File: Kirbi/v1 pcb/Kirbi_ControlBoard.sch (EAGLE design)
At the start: 69 parts, among them U1 PCA9306_LSSOP, U2 TEENSY_3.6_DIL, U3 MAX4173-SOT-23, U4 MAX4173-SOT-23, U5 LM393-8-SOIC, U6 AP2114H-1.8TRG1, U7 AP2114H-3.3TRG1

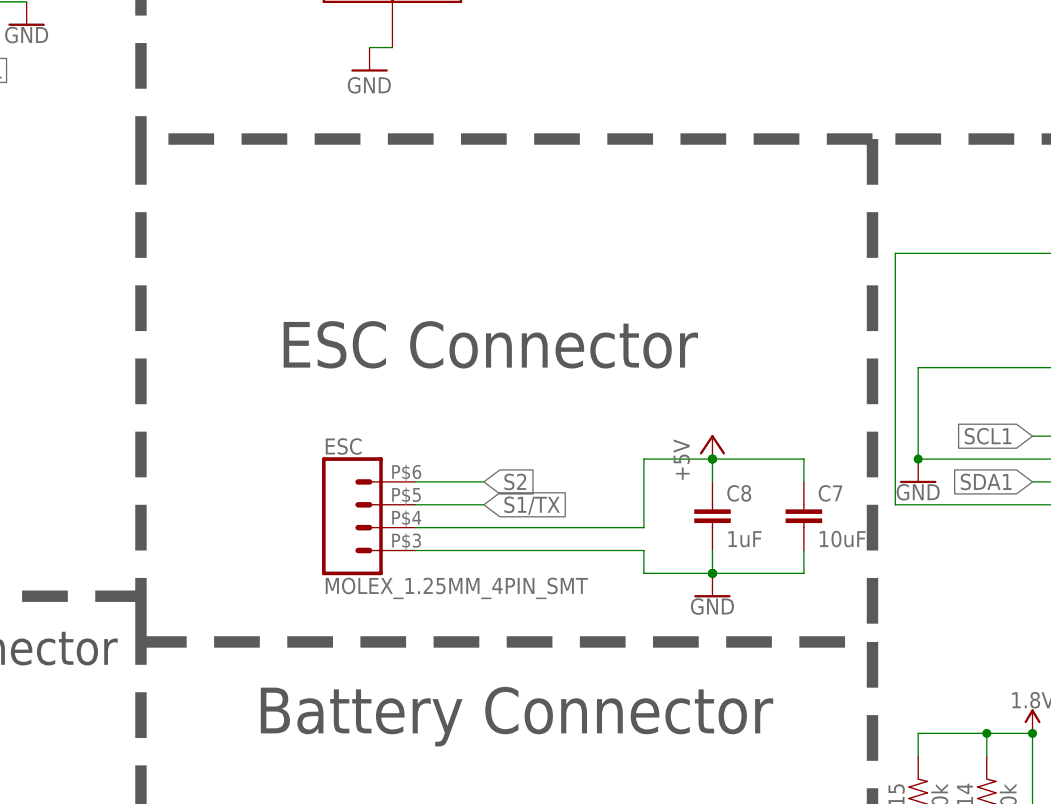
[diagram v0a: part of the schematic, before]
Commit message: Started to add power button
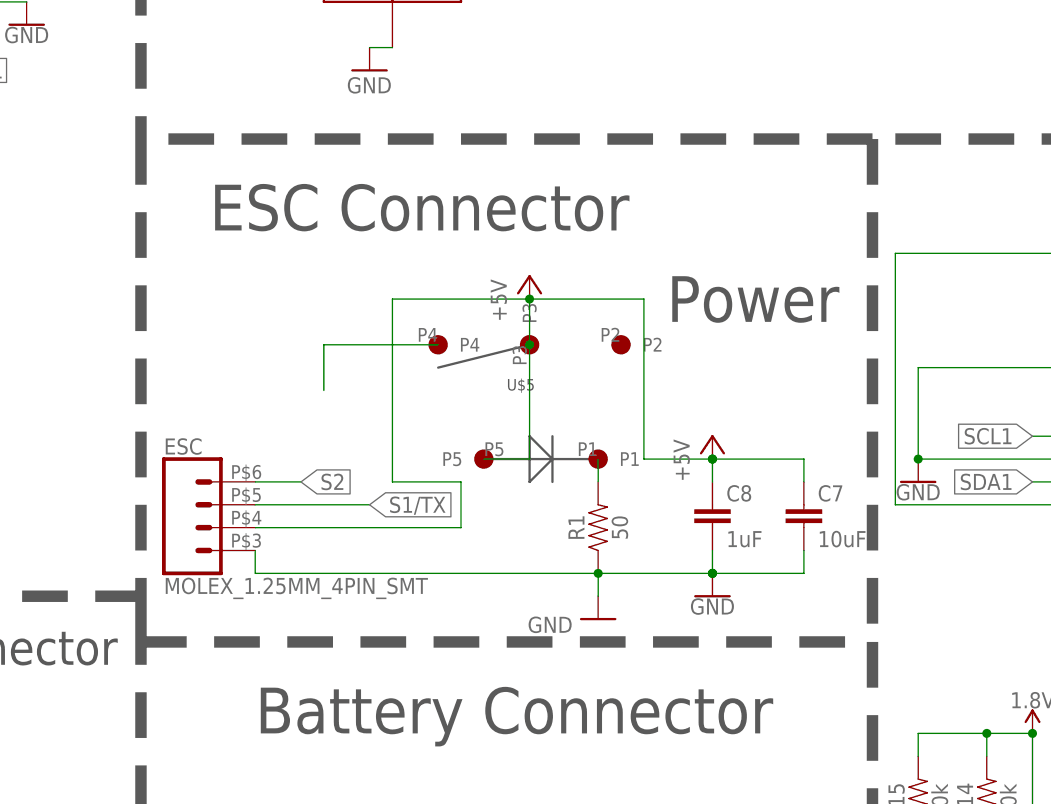
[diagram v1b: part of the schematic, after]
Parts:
- added R1: 50, SparkFun-Resistors:1KOHM-0603-1/10W-1%
- added U$5: POWER_SWITCH, Kirbi_ControlBoard:POWER_SWITCH
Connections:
- new net N$5: U$5.P4
- new net N$8: R1.2, U$5.P1
- net +5V: now also U$5.P3, U$5.P5
- net GND: now also R1.1
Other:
- note added: "Power"
- moved on the sheet: ESC
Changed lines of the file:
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@@
 <part name="LIDAR_R" library="Kirbi_ControlBoard" deviceset="MOLEX_1.25MM_4PIN_SMT" device=""/>
 <part name="LIDAR_L" library="Kirbi_ControlBoard" deviceset="MOLEX_1.25MM_4PIN_SMT" device=""/>
+<part name="U$5" library="Kirbi_ControlBoard" deviceset="POWER_SWITCH" device=""/>
+<part name="P+3" library="supply1" library_urn="urn:adsk.eagle:library:371" deviceset="+5V" device=""/>
+<part name="GND21" library="SparkFun-PowerSymbols" library_urn="urn:adsk.eagle:library:530" deviceset="GND" device=""/>
+<part name="R1" library="SparkFun-Resistors" library_urn="urn:adsk.eagle:library:532" deviceset="1KOHM" device="-0603-1/10W-1%" package3d_urn="urn:adsk.eagle:package:39650/1" value="50"/>
 </parts>
 <sheets>
@@
 <wire x1="424.18" y1="261.62" x2="424.18" y2="177.8" width="1.27" layer="97" style="shortdash"/>
 <wire x1="424.18" y1="177.8" x2="335.28" y2="177.8" width="1.27" layer="97" style="shortdash"/>
-<text x="269.24" y="152.4" size="5.08" layer="97">ESC Connector</text>
+<text x="261.62" y="167.64" size="5.08" layer="97">ESC Connector</text>
 <wire x1="335.28" y1="177.8" x2="254" y2="177.8" width="1.27" layer="97" style="shortdash"/>
 <wire x1="172.72" y1="78.74" x2="190.5" y2="78.74" width="1.27" layer="97" style="shortdash"/>
@@
 <wire x1="190.5" y1="127" x2="190.5" y2="78.74" width="1.27" layer="97" style="shortdash"/>
 <text x="185.42" y="71.12" size="5.08" layer="97">Current Sensing</text>
+<text x="312.42" y="157.48" size="5.08" layer="97">Power</text>
 </plain>
 <instances>
@@
 <attribute name="VALUE" x="340.36" y="139.446" size="1.778" layer="96" align="top-center"/>
 </instance>
-<instance part="ESC" gate="G$1" x="279.4" y="134.62" smashed="yes">
-<attribute name="VALUE" x="274.32" y="127.254" size="1.778" layer="96" font="vector"/>
-<attribute name="NAME" x="274.32" y="142.748" size="1.778" layer="95" font="vector"/>
+<instance part="ESC" gate="G$1" x="261.62" y="134.62" smashed="yes">
+<attribute name="VALUE" x="256.54" y="127.254" size="1.778" layer="96" font="vector"/>
+<attribute name="NAME" x="256.54" y="142.748" size="1.778" layer="95" font="vector"/>
 </instance>
 <instance part="LIDAR_R" gate="G$1" x="33.02" y="228.6" smashed="yes">
@@
 <attribute name="VALUE" x="66.04" y="221.234" size="1.778" layer="96" font="vector"/>
 <attribute name="NAME" x="66.04" y="236.728" size="1.778" layer="95" font="vector"/>
+</instance>
+<instance part="U$5" gate="G$1" x="297.18" y="149.86" smashed="yes">
+<attribute name="NAME" x="294.64" y="149.86" size="1.27" layer="97"/>
+</instance>
+<instance part="P+3" gate="1" x="297.18" y="162.56" smashed="yes">
+<attribute name="VALUE" x="294.64" y="157.48" size="1.778" layer="96" rot="R90"/>
+</instance>
+<instance part="GND21" gate="1" x="304.8" y="124.46" smashed="yes">
+<attribute name="VALUE" x="299.466" y="124.714" size="1.778" layer="96" align="top-center"/>
+</instance>
+<instance part="R1" gate="G$1" x="304.8" y="134.62" smashed="yes" rot="R90">
+<attribute name="NAME" x="303.276" y="134.62" size="1.778" layer="95" font="vector" rot="R90" align="bottom-center"/>
+<attribute name="VALUE" x="306.324" y="134.62" size="1.778" layer="96" font="vector" rot="R90" align="top-center"/>
 </instance>
 </instances>
@@
 <wire x1="317.5" y1="129.54" x2="327.66" y2="129.54" width="0.1524" layer="91"/>
 <junction x="317.5" y="129.54"/>
-<wire x1="284.48" y1="132.08" x2="309.88" y2="132.08" width="0.1524" layer="91"/>
-<wire x1="309.88" y1="132.08" x2="309.88" y2="129.54" width="0.1524" layer="91"/>
-<wire x1="317.5" y1="129.54" x2="309.88" y2="129.54" width="0.1524" layer="91"/>
+<wire x1="317.5" y1="129.54" x2="304.8" y2="129.54" width="0.1524" layer="91"/>
 <junction x="317.5" y="129.54"/>
+<pinref part="GND21" gate="1" pin="GND"/>
+<pinref part="R1" gate="G$1" pin="1"/>
+<wire x1="304.8" y1="127" x2="304.8" y2="129.54" width="0.1524" layer="91"/>
+<junction x="304.8" y="129.54"/>
 <pinref part="ESC" gate="G$1" pin="1"/>
+<wire x1="304.8" y1="129.54" x2="266.7" y2="129.54" width="0.1524" layer="91"/>
+<wire x1="266.7" y1="129.54" x2="266.7" y2="132.08" width="0.1524" layer="91"/>
 </segment>
 <segment>
@@
 <pinref part="P+16" gate="1" pin="+5V"/>
 <junction x="317.5" y="142.24"/>
-<wire x1="284.48" y1="134.62" x2="309.88" y2="134.62" width="0.1524" layer="91"/>
-<wire x1="309.88" y1="134.62" x2="309.88" y2="142.24" width="0.1524" layer="91"/>
 <wire x1="317.5" y1="142.24" x2="309.88" y2="142.24" width="0.1524" layer="91"/>
 <junction x="317.5" y="142.24"/>
+<pinref part="P+3" gate="1" pin="+5V"/>
+<pinref part="U$5" gate="G$1" pin="P3"/>
+<wire x1="297.18" y1="160.02" x2="297.18" y2="154.94" width="0.1524" layer="91"/>
+<pinref part="U$5" gate="G$1" pin="P5"/>
+<wire x1="297.18" y1="154.94" x2="297.18" y2="142.24" width="0.1524" layer="91"/>
+<wire x1="297.18" y1="142.24" x2="292.1" y2="142.24" width="0.1524" layer="91"/>
+<junction x="297.18" y="154.94"/>
 <pinref part="ESC" gate="G$1" pin="2"/>
+<wire x1="266.7" y1="134.62" x2="289.56" y2="134.62" width="0.1524" layer="91"/>
+<wire x1="289.56" y1="134.62" x2="289.56" y2="139.7" width="0.1524" layer="91"/>
+<wire x1="289.56" y1="139.7" x2="281.94" y2="139.7" width="0.1524" layer="91"/>
+<wire x1="281.94" y1="139.7" x2="281.94" y2="160.02" width="0.1524" layer="91"/>
+<wire x1="281.94" y1="160.02" x2="297.18" y2="160.02" width="0.1524" layer="91"/>
+<junction x="297.18" y="160.02"/>
+<wire x1="309.88" y1="142.24" x2="309.88" y2="160.02" width="0.1524" layer="91"/>
+<wire x1="309.88" y1="160.02" x2="297.18" y2="160.02" width="0.1524" layer="91"/>
 </segment>
 <segment>
@@
 <net name="S1/TX" class="0">
 <segment>
-<wire x1="284.48" y1="137.16" x2="292.1" y2="137.16" width="0.1524" layer="91"/>
-<label x="292.1" y="137.16" size="1.778" layer="95" xref="yes"/>
+<wire x1="266.7" y1="137.16" x2="279.4" y2="137.16" width="0.1524" layer="91"/>
+<label x="279.4" y="137.16" size="1.778" layer="95" xref="yes"/>
 <pinref part="ESC" gate="G$1" pin="3"/>
 </segment>
@@
 <net name="S2" class="0">
 <segment>
-<wire x1="284.48" y1="139.7" x2="292.1" y2="139.7" width="0.1524" layer="91"/>
-<label x="292.1" y="139.7" size="1.778" layer="95" xref="yes"/>
+<wire x1="266.7" y1="139.7" x2="271.78" y2="139.7" width="0.1524" layer="91"/>
+<label x="271.78" y="139.7" size="1.778" layer="95" xref="yes"/>
 <pinref part="ESC" gate="G$1" pin="4"/>
 </segment>
@@
 </segment>
 </net>
+<net name="N$5" class="0">
+<segment>
+<pinref part="U$5" gate="G$1" pin="P4"/>
+<wire x1="287.02" y1="154.94" x2="274.32" y2="154.94" width="0.1524" layer="91"/>
+<wire x1="274.32" y1="154.94" x2="274.32" y2="149.86" width="0.1524" layer="91"/>
+</segment>
+</net>
+<net name="N$8" class="0">
+<segment>
+<pinref part="U$5" gate="G$1" pin="P1"/>
+<pinref part="R1" gate="G$1" pin="2"/>
+<wire x1="304.8" y1="139.7" x2="304.8" y2="142.24" width="0.1524" layer="91"/>
+</segment>
+</net>
